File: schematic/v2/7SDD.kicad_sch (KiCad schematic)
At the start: 6 parts, among them U18 HDSP-7503, U19 HDSP-7503, U2 HDSP-7503, U4 YAAJ_BluePill_Part_Like

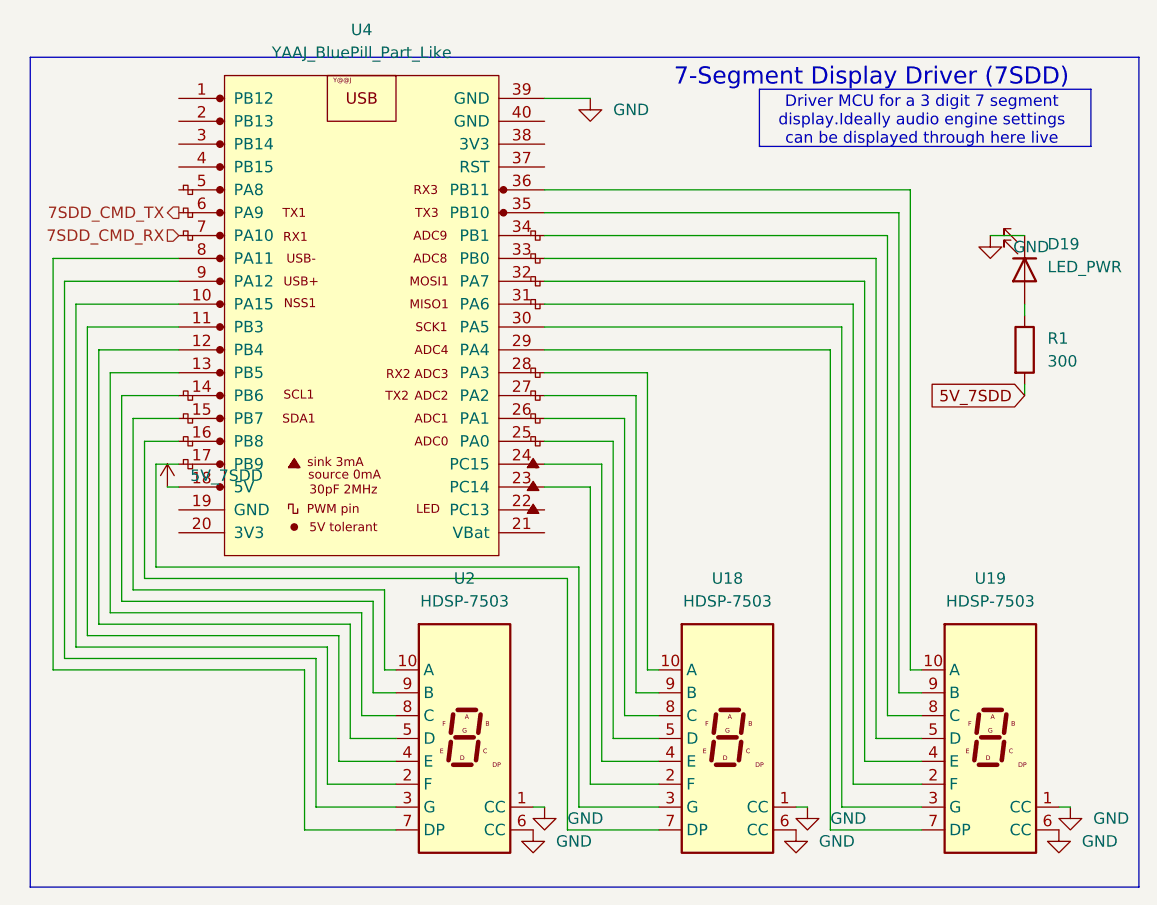
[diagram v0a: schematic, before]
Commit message: no errors in the ERC!
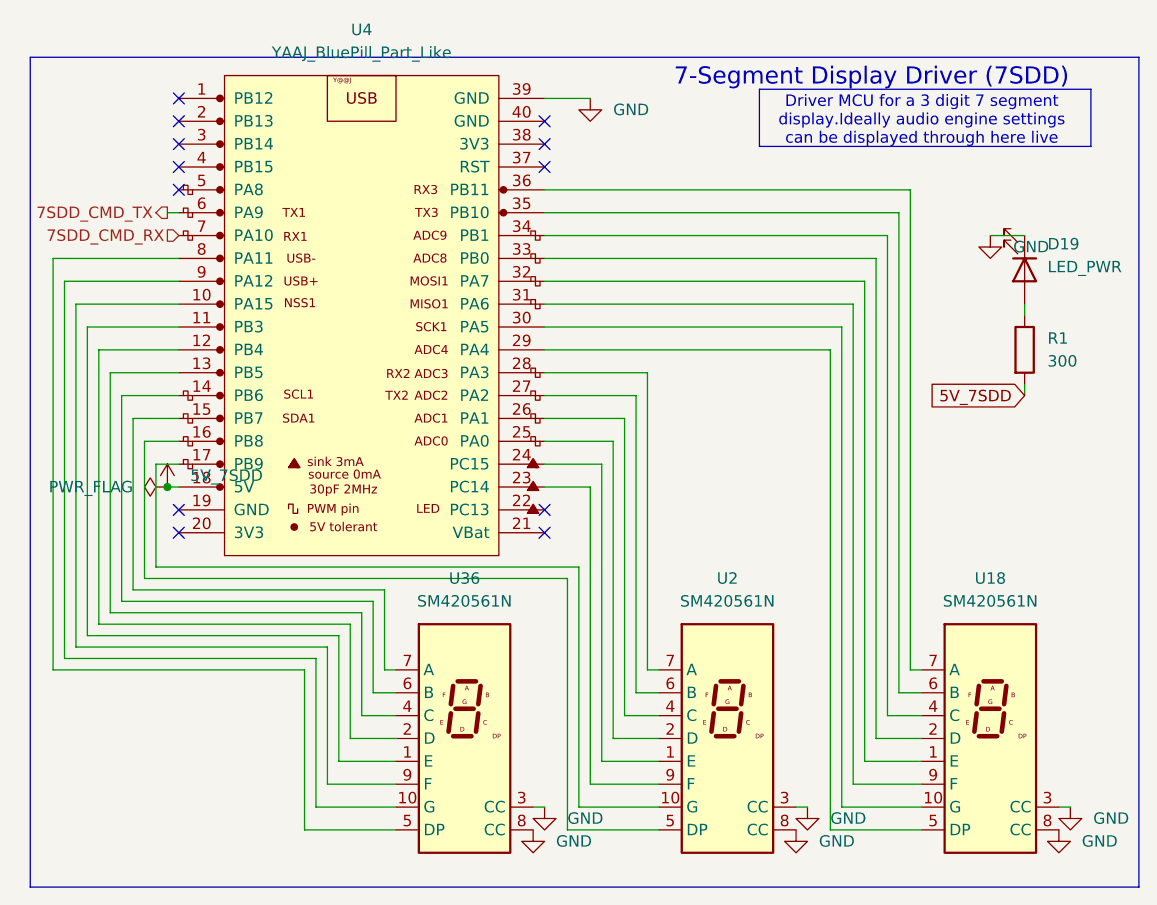
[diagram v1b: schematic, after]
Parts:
- removed U18, U19, U2: HDSP-7503, Display_7Segment:HDSP-A151, symbol Display_Character:HDSP-7503
- added U18, U2, U36: SM420561N, Display_7Segment:7SegmentLED_LTS6760_LTS6780, symbol Display_Character:SM420561N
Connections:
- net GND: now also U18.3 (CC), U18.8 (CC), U2.3 (CC), U2.8 (CC), U36.3 (CC), U36.8 (CC)
- net at U4.36 (PB11): now also U18.7 (A)
- net at U4.31 (PA6): now also U18.9 (F)
- net at U4.30 (PA5): now also U18.10 (G)
- net at U4.32 (PA7): now also U18.1 (E)
- net at U4.33 (PB0): now also U18.2 (D)
- net at U4.29 (PA4): now also U18.5 (DP)
- net at U4.34 (PB1): now also U18.4 (C)
- net at U4.35 (PB10): now also U18.6 (B)
- net at U4.28 (PA3): now also U2.7 (A)
- net at U4.23 (PC14): now also U2.9 (F)
- net at U4.17 (PB9): now also U2.10 (G)
- net at U4.24 (PC15): now also U2.1 (E)
- net at U4.25 (PA0): now also U2.2 (D)
- net at U4.16 (PB8): now also U2.5 (DP)
- net at U4.26 (PA1): now also U2.4 (C)
- net at U4.27 (PA2): now also U2.6 (B)
- net at U4.15 (PB7): now also U36.7 (A)
- net at U4.10 (PA15): now also U36.9 (F)
- net at U4.9 (PA12): now also U36.10 (G)
- net at U4.11 (PB3): now also U36.1 (E)
- net at U4.12 (PB4): now also U36.2 (D)
- net at U4.8 (PA11): now also U36.5 (DP)
- net at U4.13 (PB5): now also U36.4 (C)
- net at U4.14 (PB6): now also U36.6 (B)
- no-connect marks 0 -> 12
